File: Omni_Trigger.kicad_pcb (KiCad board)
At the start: 2 copper layers, 121.2 x 47.8 mm, 43 parts, among them J1 Screw_Terminal_01x02, J2 Screw_Terminal_01x02, J3 Conn_02x13_Top_Bottom, J4 Conn_02x04_Odd_Even, J5 Conn_02x02_Odd_Even, J6 Conn_02x04_Odd_Even, J7 Screw_Terminal_01x08, J8 Screw_Terminal_01x04, K1 G5LE-1, K2 G5LE-1, K3 G5LE-1, K4 G5LE-1, Q1 BS170F, Q2 BS170F, Q3 BS170F, Q4 BS170F

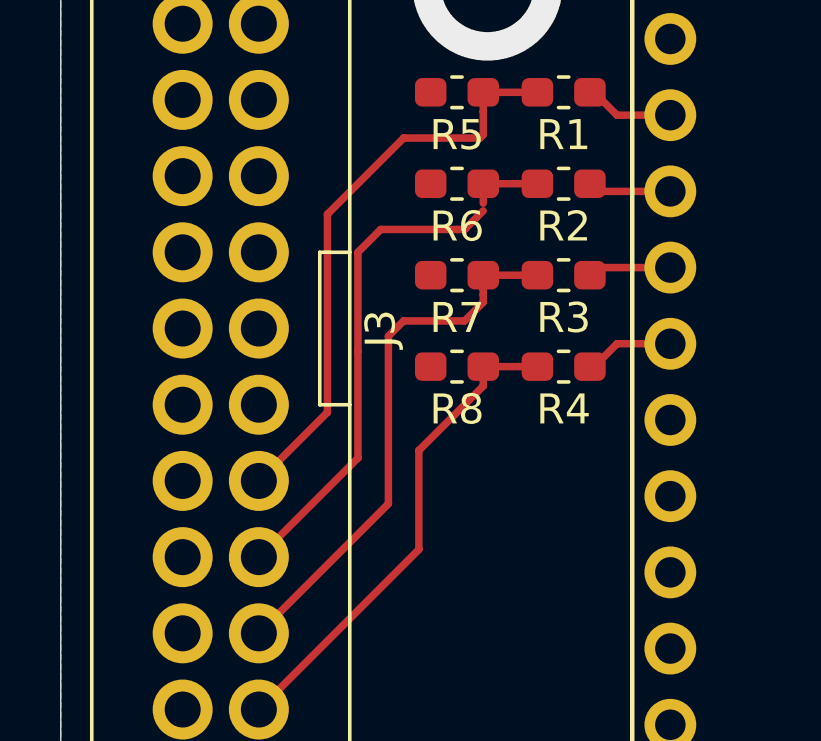
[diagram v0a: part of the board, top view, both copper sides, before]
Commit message: Updated clearances
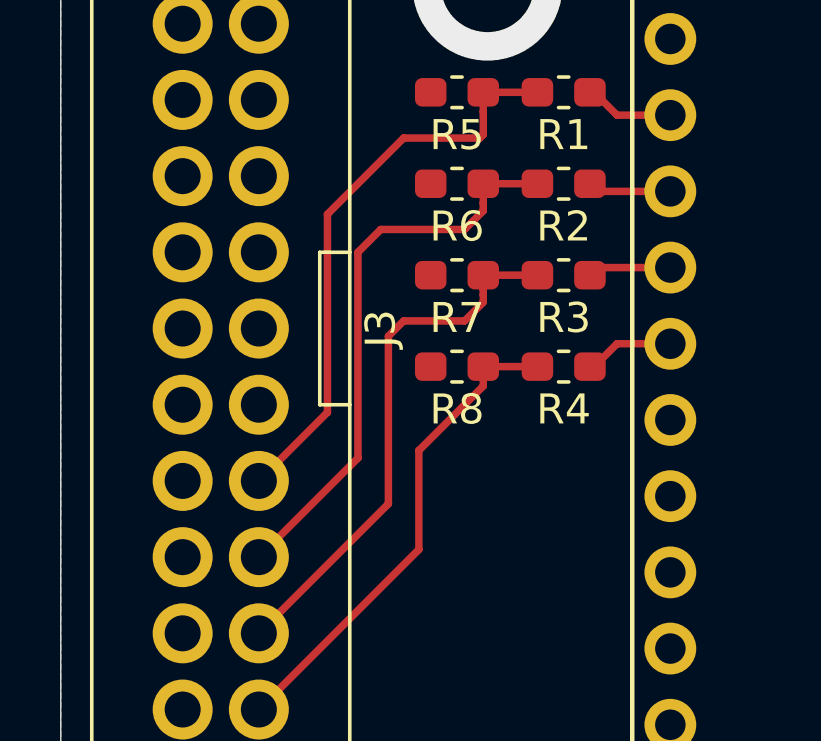
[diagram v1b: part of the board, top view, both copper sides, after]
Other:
- net class Default: clearance 0.2 -> 0.15
- net class Signal: clearance 0.2 -> 0.65
- rule trace_clearance: 0.2 -> 0.15
